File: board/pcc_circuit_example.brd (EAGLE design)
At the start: 47.5 x 29.1 mm, 18 parts, among them T1 BT138-V

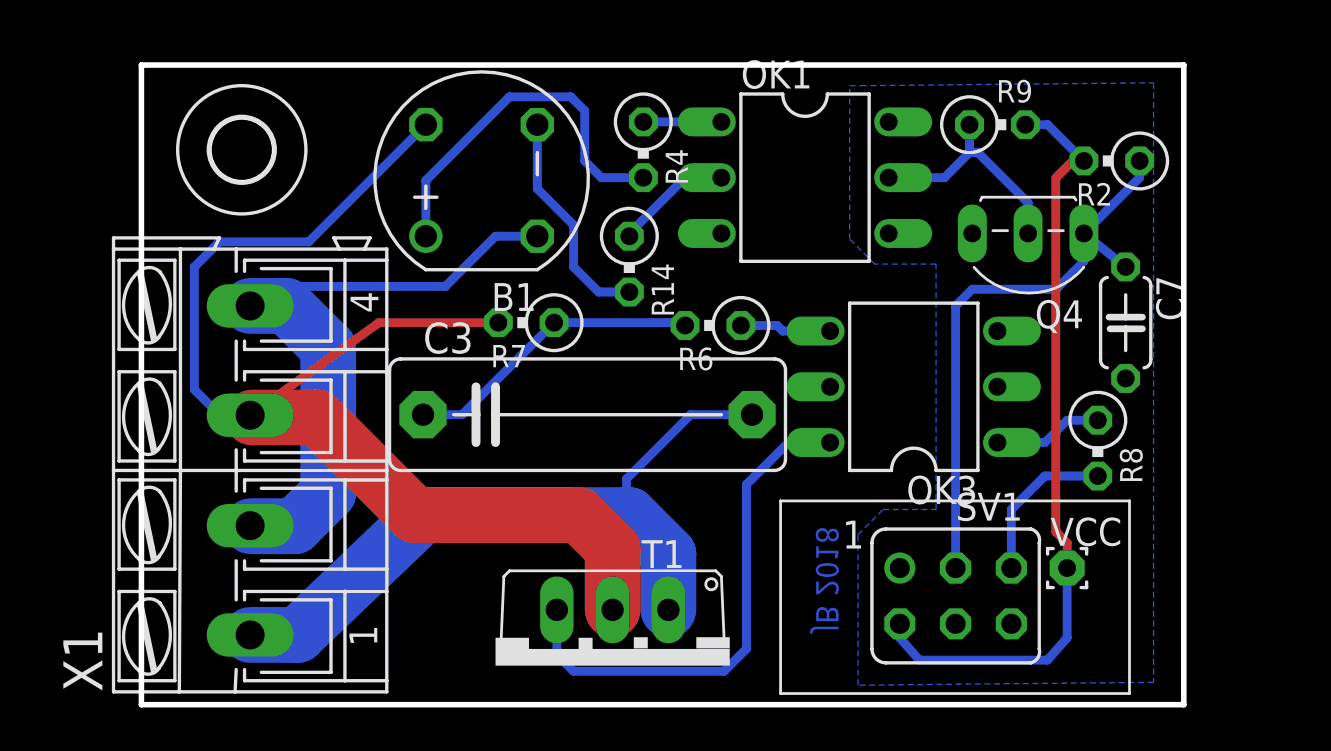
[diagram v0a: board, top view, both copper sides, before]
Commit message: a bit more space..
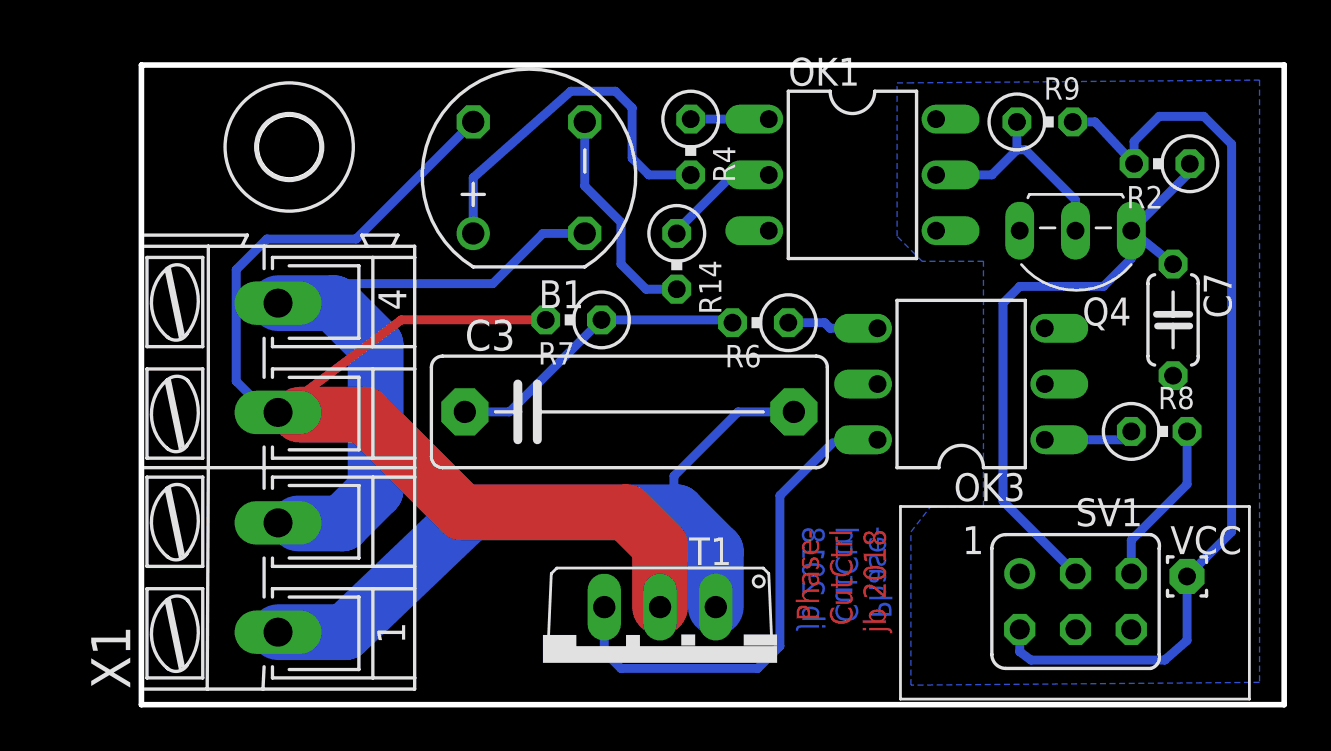
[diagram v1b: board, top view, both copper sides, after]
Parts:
- moved VCC 5.47 mm to (47.6, 5.84)
- moved SV1 5.47 mm to (42.5, 4.70)
- moved R8 2.90 mm to (46.4, 12.4), turned to 0 degrees
- moved R2 2.29 mm to (46.5, 24.6)
- moved R9 2.16 mm to (41.1, 26.5)
- moved U$3 2.16 mm to (6.73, 25.4)
- moved B1 2.16 mm to (17.7, 24.0)
- moved C7 2.16 mm to (47.0, 17.5)
- moved OK1 2.16 mm to (32.4, 24.1)
- moved OK3 2.16 mm to (37.3, 14.6)
- moved Q4 2.16 mm to (42.5, 20.3)
- moved R14 2.16 mm to (24.4, 20.2)
- moved R4 2.16 mm to (25.0, 25.4)
- moved R6 2.16 mm to (28.2, 17.4)
- moved R7 2.16 mm to (19.7, 17.5)
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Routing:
- net VCC: track 35.3 -> 42.6 mm
- net AC220V1: track 29.5 -> 32.0 mm
- net AC220V2: track 54.9 -> 56.9 mm
- net ATMEGA-PIN3: track 26.7 -> 28.2 mm
- net N$11: track 4.99 -> 4.09 mm
- net 220V_LOAD: track 35.5 -> 36.1 mm
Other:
- board size 47.5 x 29.1 mm -> 52 x 29.1 mm
- board text added: "Phase- CutCtrl jb 2018"
- board text removed: "JB 2018"
